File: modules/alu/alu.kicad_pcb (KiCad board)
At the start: 2 copper layers, 95 parts, among them Q1 2N3904, Q10 2N3906, Q11 2N3904, Q12 2N3904, Q13 2N3904, Q14 2N3904, Q15 2N3904, Q16 2N3904, Q17 2N3904, Q18 2N3906, Q19 2N3904, Q2 2N3904, Q20 2N3906, Q21 2N3904, Q22 2N3906, Q23 2N3904, Q24 2N3906, Q25 2N3906, Q26 2N3906, Q27 2N3906, Q28 2N3904, Q29 2N3904, Q3 2N3904, Q30 2N3904, Q31 2N3906, Q32 2N3906, Q33 2N3904, Q34 2N3904, Q35 2N3906, Q36 2N3904, Q37 2N3906, Q38 2N3906, Q39 2N3906, Q4 2N3904, Q40 2N3906, Q41 2N3906, Q42 2N3906, Q43 2N3904, Q44 2N3904, Q45 2N3904, Q5 2N3904, Q6 2N3904, Q7 2N3906, Q8 2N3906, Q9 2N3906

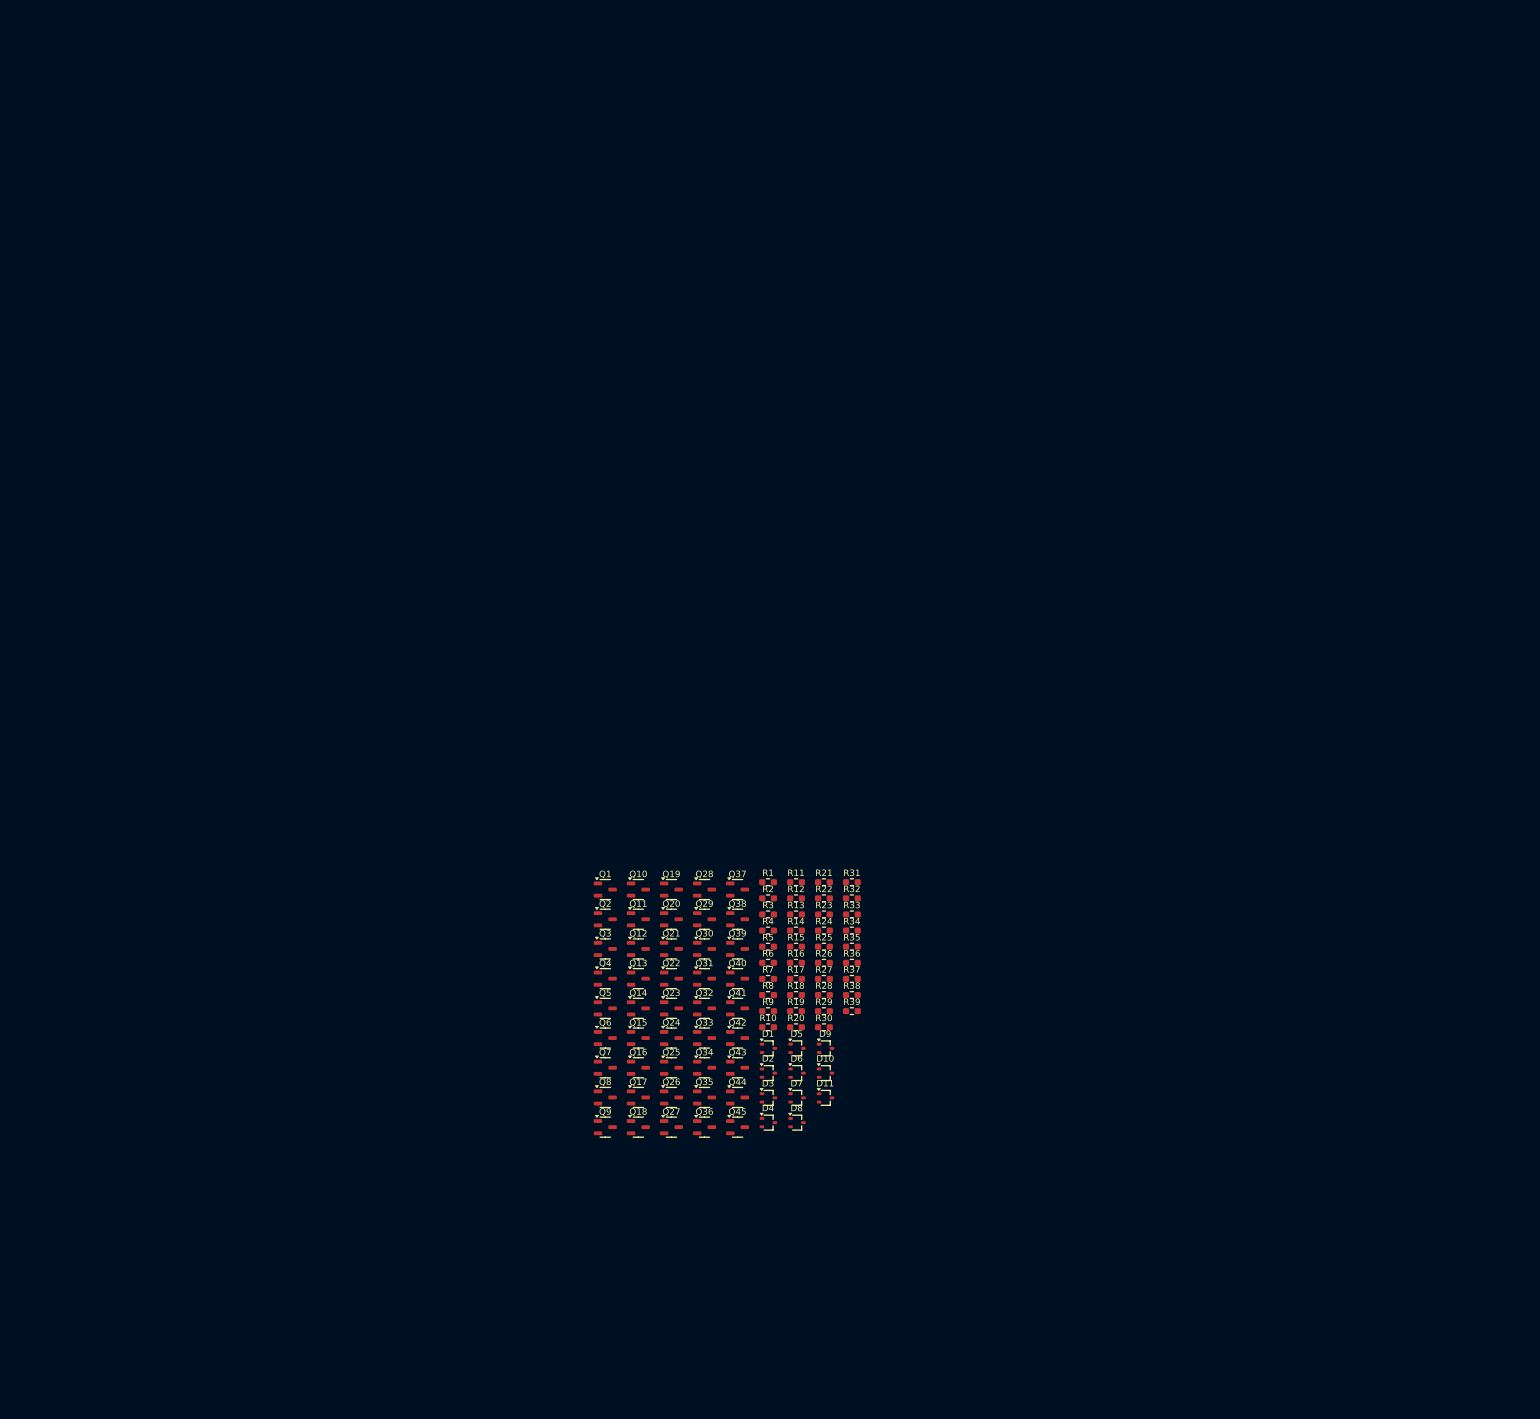
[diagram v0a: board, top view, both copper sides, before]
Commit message: Small ALU fix.
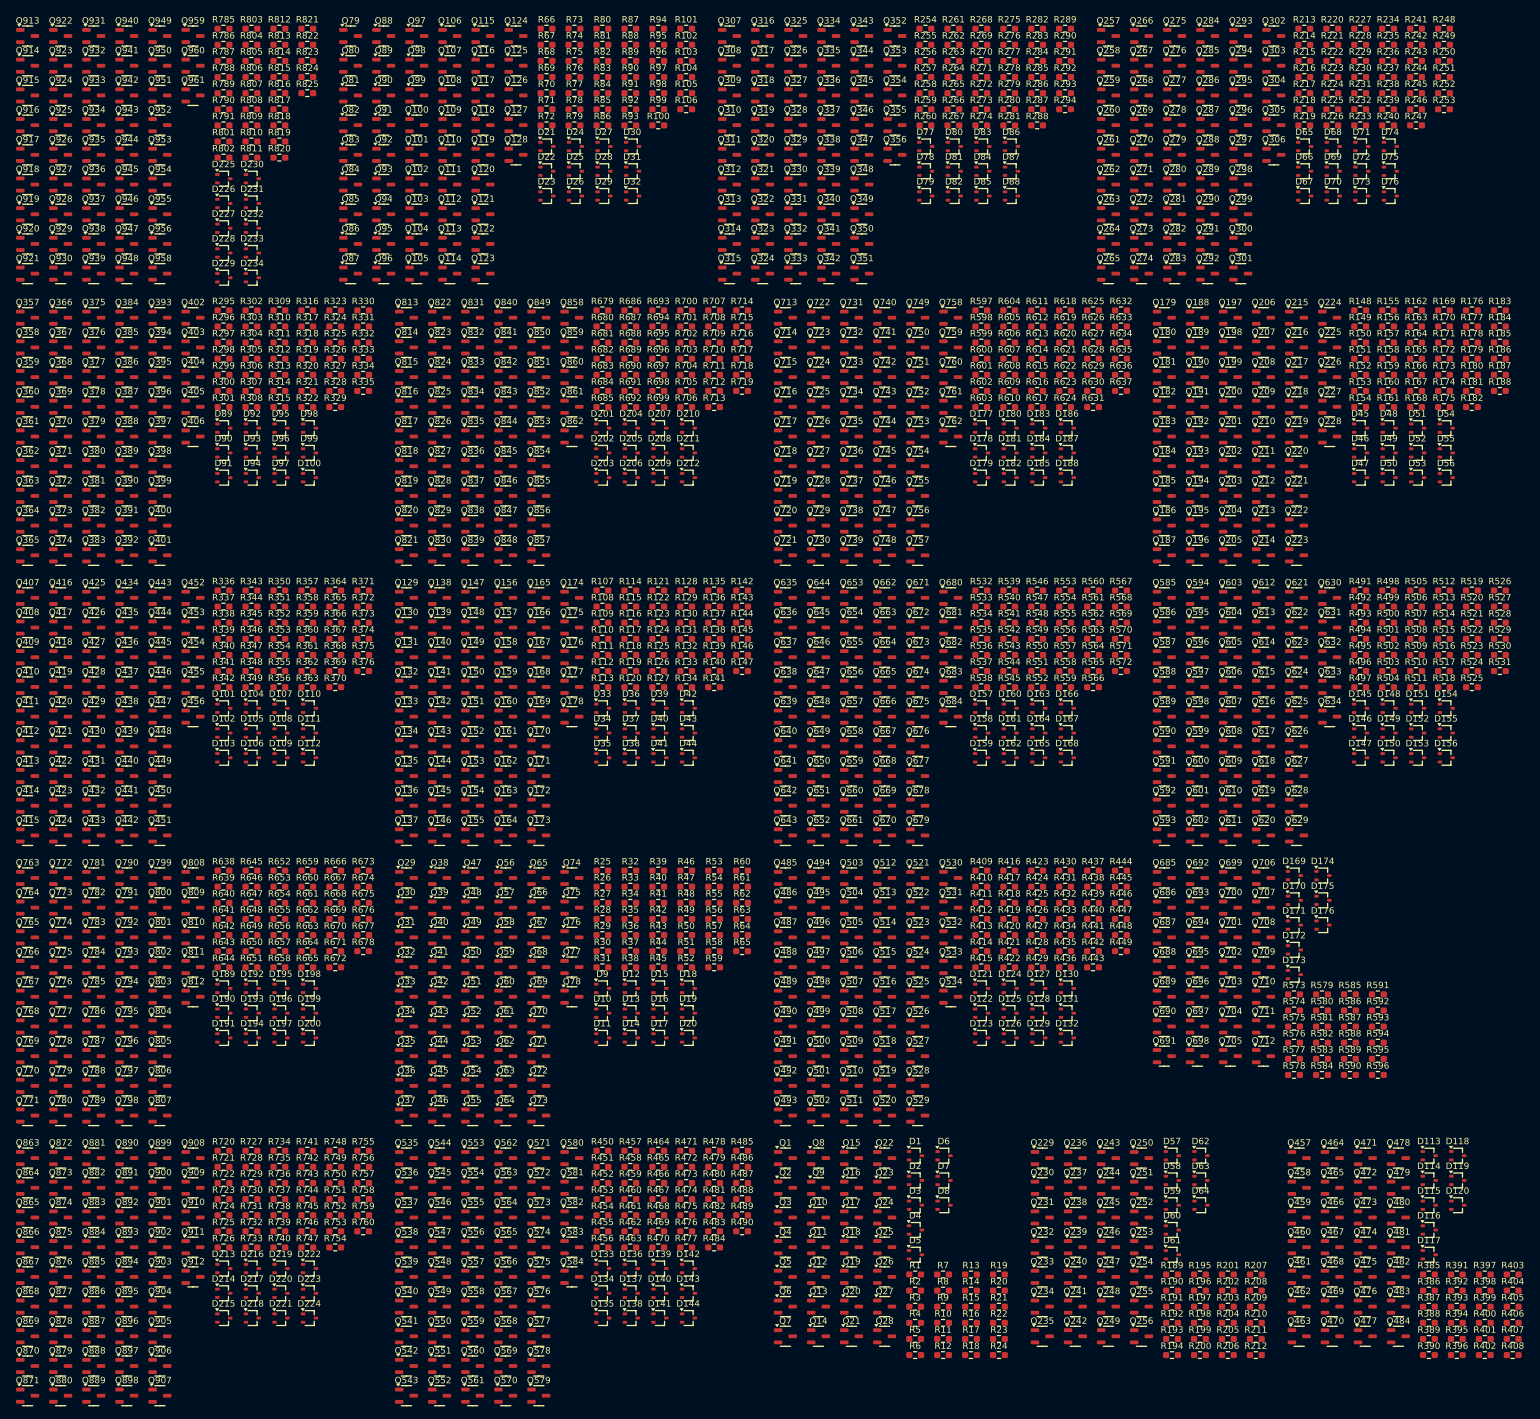
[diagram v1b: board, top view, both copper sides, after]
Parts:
- added D100: BAT54W, Package_TO_SOT_SMD:SOT-323_SC-70, F.Cu at (73.8, 3.92)
- added D101: BAT54W, Package_TO_SOT_SMD:SOT-323_SC-70, F.Cu at (60.5, 39.8)
- added D102: BAT54W, Package_TO_SOT_SMD:SOT-323_SC-70, F.Cu at (60.5, 43.7)
- added D103: BAT54W, Package_TO_SOT_SMD:SOT-323_SC-70, F.Cu at (60.5, 47.5)
- added D104: BAT54W, Package_TO_SOT_SMD:SOT-323_SC-70, F.Cu at (65.0, 39.8)
- added D105: BAT54W, Package_TO_SOT_SMD:SOT-323_SC-70, F.Cu at (65.0, 43.7)
- added D106: BAT54W, Package_TO_SOT_SMD:SOT-323_SC-70, F.Cu at (65.0, 47.5)
- added D107: BAT54W, Package_TO_SOT_SMD:SOT-323_SC-70, F.Cu at (69.4, 39.8)
- added D108: BAT54W, Package_TO_SOT_SMD:SOT-323_SC-70, F.Cu at (69.4, 43.7)
- added D109: BAT54W, Package_TO_SOT_SMD:SOT-323_SC-70, F.Cu at (69.4, 47.5)
- added D110: BAT54W, Package_TO_SOT_SMD:SOT-323_SC-70, F.Cu at (73.8, 39.8)
- added D111: BAT54W, Package_TO_SOT_SMD:SOT-323_SC-70, F.Cu at (73.8, 43.7)
- added D112: BAT54W, Package_TO_SOT_SMD:SOT-323_SC-70, F.Cu at (73.8, 47.5)
- added D113: BAT54W, Package_TO_SOT_SMD:SOT-323_SC-70, F.Cu at (248.2, 109.5)
- added D114: BAT54W, Package_TO_SOT_SMD:SOT-323_SC-70, F.Cu at (248.2, 113.4)
- added D115: BAT54W, Package_TO_SOT_SMD:SOT-323_SC-70, F.Cu at (248.2, 117.2)
- added D116: BAT54W, Package_TO_SOT_SMD:SOT-323_SC-70, F.Cu at (248.2, 121.1)
- added D117: BAT54W, Package_TO_SOT_SMD:SOT-323_SC-70, F.Cu at (248.2, 124.9)
- added D118: BAT54W, Package_TO_SOT_SMD:SOT-323_SC-70, F.Cu at (252.7, 109.5)
- added D119: BAT54W, Package_TO_SOT_SMD:SOT-323_SC-70, F.Cu at (252.7, 113.4)
- added D12: BAT54W, Package_TO_SOT_SMD:SOT-323_SC-70, F.Cu at (124.0, 83.5)
- added D120: BAT54W, Package_TO_SOT_SMD:SOT-323_SC-70, F.Cu at (252.7, 117.2)
- added D121: BAT54W, Package_TO_SOT_SMD:SOT-323_SC-70, F.Cu at (178.5, 83.5)
- added D122: BAT54W, Package_TO_SOT_SMD:SOT-323_SC-70, F.Cu at (178.5, 87.3)
- added D123: BAT54W, Package_TO_SOT_SMD:SOT-323_SC-70, F.Cu at (178.5, 91.2)
- added D124: BAT54W, Package_TO_SOT_SMD:SOT-323_SC-70, F.Cu at (182.9, 83.5)
- added D125: BAT54W, Package_TO_SOT_SMD:SOT-323_SC-70, F.Cu at (182.9, 87.3)
- added D126: BAT54W, Package_TO_SOT_SMD:SOT-323_SC-70, F.Cu at (182.9, 91.2)
- added D127: BAT54W, Package_TO_SOT_SMD:SOT-323_SC-70, F.Cu at (187.4, 83.5)
- added D128: BAT54W, Package_TO_SOT_SMD:SOT-323_SC-70, F.Cu at (187.4, 87.3)
- added D129: BAT54W, Package_TO_SOT_SMD:SOT-323_SC-70, F.Cu at (187.4, 91.2)
- added D13: BAT54W, Package_TO_SOT_SMD:SOT-323_SC-70, F.Cu at (124.0, 87.3)
- added D130: BAT54W, Package_TO_SOT_SMD:SOT-323_SC-70, F.Cu at (191.8, 83.5)
- added D131: BAT54W, Package_TO_SOT_SMD:SOT-323_SC-70, F.Cu at (191.8, 87.3)
- added D132: BAT54W, Package_TO_SOT_SMD:SOT-323_SC-70, F.Cu at (191.8, 91.2)
- added D133: BAT54W, Package_TO_SOT_SMD:SOT-323_SC-70, F.Cu at (119.5, 127.1)
- added D134: BAT54W, Package_TO_SOT_SMD:SOT-323_SC-70, F.Cu at (119.5, 130.9)
- added D135: BAT54W, Package_TO_SOT_SMD:SOT-323_SC-70, F.Cu at (119.5, 134.8)
- added D136: BAT54W, Package_TO_SOT_SMD:SOT-323_SC-70, F.Cu at (124.0, 127.1)
- added D137: BAT54W, Package_TO_SOT_SMD:SOT-323_SC-70, F.Cu at (124.0, 130.9)
- added D138: BAT54W, Package_TO_SOT_SMD:SOT-323_SC-70, F.Cu at (124.0, 134.8)
- added D139: BAT54W, Package_TO_SOT_SMD:SOT-323_SC-70, F.Cu at (128.4, 127.1)
- added D14: BAT54W, Package_TO_SOT_SMD:SOT-323_SC-70, F.Cu at (124.0, 91.2)
- added D140: BAT54W, Package_TO_SOT_SMD:SOT-323_SC-70, F.Cu at (128.4, 130.9)
- added D141: BAT54W, Package_TO_SOT_SMD:SOT-323_SC-70, F.Cu at (128.4, 134.8)
- added D142: BAT54W, Package_TO_SOT_SMD:SOT-323_SC-70, F.Cu at (132.8, 127.1)
- added D143: BAT54W, Package_TO_SOT_SMD:SOT-323_SC-70, F.Cu at (132.8, 130.9)
- added D144: BAT54W, Package_TO_SOT_SMD:SOT-323_SC-70, F.Cu at (132.8, 134.8)
- added D145: BAT54W, Package_TO_SOT_SMD:SOT-323_SC-70, F.Cu at (237.5, 39.8)
- added D146: BAT54W, Package_TO_SOT_SMD:SOT-323_SC-70, F.Cu at (237.5, 43.7)
- added D147: BAT54W, Package_TO_SOT_SMD:SOT-323_SC-70, F.Cu at (237.5, 47.5)
- added D148: BAT54W, Package_TO_SOT_SMD:SOT-323_SC-70, F.Cu at (241.9, 39.8)
- added D149: BAT54W, Package_TO_SOT_SMD:SOT-323_SC-70, F.Cu at (241.9, 43.7)
- added D15: BAT54W, Package_TO_SOT_SMD:SOT-323_SC-70, F.Cu at (128.4, 83.5)
- added D150: BAT54W, Package_TO_SOT_SMD:SOT-323_SC-70, F.Cu at (241.9, 47.5)
- added D151: BAT54W, Package_TO_SOT_SMD:SOT-323_SC-70, F.Cu at (246.4, 39.8)
- added D152: BAT54W, Package_TO_SOT_SMD:SOT-323_SC-70, F.Cu at (246.4, 43.7)
- added D153: BAT54W, Package_TO_SOT_SMD:SOT-323_SC-70, F.Cu at (246.4, 47.5)
- added D154: BAT54W, Package_TO_SOT_SMD:SOT-323_SC-70, F.Cu at (250.8, 39.8)
- added D155: BAT54W, Package_TO_SOT_SMD:SOT-323_SC-70, F.Cu at (250.8, 43.7)
- added D156: BAT54W, Package_TO_SOT_SMD:SOT-323_SC-70, F.Cu at (250.8, 47.5)
- added D157: BAT54W, Package_TO_SOT_SMD:SOT-323_SC-70, F.Cu at (178.5, 39.8)
- added D158: BAT54W, Package_TO_SOT_SMD:SOT-323_SC-70, F.Cu at (178.5, 43.7)
- added D159: BAT54W, Package_TO_SOT_SMD:SOT-323_SC-70, F.Cu at (178.5, 47.5)
- added D16: BAT54W, Package_TO_SOT_SMD:SOT-323_SC-70, F.Cu at (128.4, 87.3)
- added D160: BAT54W, Package_TO_SOT_SMD:SOT-323_SC-70, F.Cu at (182.9, 39.8)
- added D161: BAT54W, Package_TO_SOT_SMD:SOT-323_SC-70, F.Cu at (182.9, 43.7)
- added D162: BAT54W, Package_TO_SOT_SMD:SOT-323_SC-70, F.Cu at (182.9, 47.5)
- added D163: BAT54W, Package_TO_SOT_SMD:SOT-323_SC-70, F.Cu at (187.4, 39.8)
- added D164: BAT54W, Package_TO_SOT_SMD:SOT-323_SC-70, F.Cu at (187.4, 43.7)
- added D165: BAT54W, Package_TO_SOT_SMD:SOT-323_SC-70, F.Cu at (187.4, 47.5)
- added D166: BAT54W, Package_TO_SOT_SMD:SOT-323_SC-70, F.Cu at (191.8, 39.8)
- added D167: BAT54W, Package_TO_SOT_SMD:SOT-323_SC-70, F.Cu at (191.8, 43.7)
- added D168: BAT54W, Package_TO_SOT_SMD:SOT-323_SC-70, F.Cu at (191.8, 47.5)
- added D169: BAT54W, Package_TO_SOT_SMD:SOT-323_SC-70, F.Cu at (227.2, 65.9)
- added D17: BAT54W, Package_TO_SOT_SMD:SOT-323_SC-70, F.Cu at (128.4, 91.2)
- added D170: BAT54W, Package_TO_SOT_SMD:SOT-323_SC-70, F.Cu at (227.2, 69.7)
- added D171: BAT54W, Package_TO_SOT_SMD:SOT-323_SC-70, F.Cu at (227.2, 73.6)
- added D172: BAT54W, Package_TO_SOT_SMD:SOT-323_SC-70, F.Cu at (227.2, 77.5)
- added D173: BAT54W, Package_TO_SOT_SMD:SOT-323_SC-70, F.Cu at (227.2, 81.3)
- added D174: BAT54W, Package_TO_SOT_SMD:SOT-323_SC-70, F.Cu at (231.7, 65.9)
- added D175: BAT54W, Package_TO_SOT_SMD:SOT-323_SC-70, F.Cu at (231.7, 69.7)
- added D176: BAT54W, Package_TO_SOT_SMD:SOT-323_SC-70, F.Cu at (231.7, 73.6)
- added D177: BAT54W, Package_TO_SOT_SMD:SOT-323_SC-70, F.Cu at (178.5, -3.79)
- added D178: BAT54W, Package_TO_SOT_SMD:SOT-323_SC-70, F.Cu at (178.5, 0.07)
- added D179: BAT54W, Package_TO_SOT_SMD:SOT-323_SC-70, F.Cu at (178.5, 3.92)
- added D18: BAT54W, Package_TO_SOT_SMD:SOT-323_SC-70, F.Cu at (132.8, 83.5)
- added D180: BAT54W, Package_TO_SOT_SMD:SOT-323_SC-70, F.Cu at (182.9, -3.79)
- added D181: BAT54W, Package_TO_SOT_SMD:SOT-323_SC-70, F.Cu at (182.9, 0.07)
- added D182: BAT54W, Package_TO_SOT_SMD:SOT-323_SC-70, F.Cu at (182.9, 3.92)
- added D183: BAT54W, Package_TO_SOT_SMD:SOT-323_SC-70, F.Cu at (187.4, -3.79)
- added D184: BAT54W, Package_TO_SOT_SMD:SOT-323_SC-70, F.Cu at (187.4, 0.07)
- added D185: BAT54W, Package_TO_SOT_SMD:SOT-323_SC-70, F.Cu at (187.4, 3.92)
- added D186: BAT54W, Package_TO_SOT_SMD:SOT-323_SC-70, F.Cu at (191.8, -3.79)
- added D187: BAT54W, Package_TO_SOT_SMD:SOT-323_SC-70, F.Cu at (191.8, 0.07)
- added D188: BAT54W, Package_TO_SOT_SMD:SOT-323_SC-70, F.Cu at (191.8, 3.92)
- added D189: BAT54W, Package_TO_SOT_SMD:SOT-323_SC-70, F.Cu at (60.5, 83.5)
- added D19: BAT54W, Package_TO_SOT_SMD:SOT-323_SC-70, F.Cu at (132.8, 87.3)
- added D190: BAT54W, Package_TO_SOT_SMD:SOT-323_SC-70, F.Cu at (60.5, 87.3)
- added D191: BAT54W, Package_TO_SOT_SMD:SOT-323_SC-70, F.Cu at (60.5, 91.2)
- added D192: BAT54W, Package_TO_SOT_SMD:SOT-323_SC-70, F.Cu at (65.0, 83.5)
- added D193: BAT54W, Package_TO_SOT_SMD:SOT-323_SC-70, F.Cu at (65.0, 87.3)
- added D194: BAT54W, Package_TO_SOT_SMD:SOT-323_SC-70, F.Cu at (65.0, 91.2)
- added D195: BAT54W, Package_TO_SOT_SMD:SOT-323_SC-70, F.Cu at (69.4, 83.5)
- added D196: BAT54W, Package_TO_SOT_SMD:SOT-323_SC-70, F.Cu at (69.4, 87.3)
- added D197: BAT54W, Package_TO_SOT_SMD:SOT-323_SC-70, F.Cu at (69.4, 91.2)
- added D198: BAT54W, Package_TO_SOT_SMD:SOT-323_SC-70, F.Cu at (73.8, 83.5)
- added D199: BAT54W, Package_TO_SOT_SMD:SOT-323_SC-70, F.Cu at (73.8, 87.3)
- added D20: BAT54W, Package_TO_SOT_SMD:SOT-323_SC-70, F.Cu at (132.8, 91.2)
- added D200: BAT54W, Package_TO_SOT_SMD:SOT-323_SC-70, F.Cu at (73.8, 91.2)
- added D201: BAT54W, Package_TO_SOT_SMD:SOT-323_SC-70, F.Cu at (119.5, -3.79)
- added D202: BAT54W, Package_TO_SOT_SMD:SOT-323_SC-70, F.Cu at (119.5, 0.07)
- added D203: BAT54W, Package_TO_SOT_SMD:SOT-323_SC-70, F.Cu at (119.5, 3.92)
- added D204: BAT54W, Package_TO_SOT_SMD:SOT-323_SC-70, F.Cu at (124.0, -3.79)
- added D205: BAT54W, Package_TO_SOT_SMD:SOT-323_SC-70, F.Cu at (124.0, 0.07)
- added D206: BAT54W, Package_TO_SOT_SMD:SOT-323_SC-70, F.Cu at (124.0, 3.92)
- added D207: BAT54W, Package_TO_SOT_SMD:SOT-323_SC-70, F.Cu at (128.4, -3.79)
- added D208: BAT54W, Package_TO_SOT_SMD:SOT-323_SC-70, F.Cu at (128.4, 0.07)
- added D209: BAT54W, Package_TO_SOT_SMD:SOT-323_SC-70, F.Cu at (128.4, 3.92)
- added D21: BAT54W, Package_TO_SOT_SMD:SOT-323_SC-70, F.Cu at (110.8, -47.6)
- added D210: BAT54W, Package_TO_SOT_SMD:SOT-323_SC-70, F.Cu at (132.8, -3.79)
- added D211: BAT54W, Package_TO_SOT_SMD:SOT-323_SC-70, F.Cu at (132.8, 0.07)
- added D212: BAT54W, Package_TO_SOT_SMD:SOT-323_SC-70, F.Cu at (132.8, 3.92)
- added D213: BAT54W, Package_TO_SOT_SMD:SOT-323_SC-70, F.Cu at (60.5, 127.1)
- added D214: BAT54W, Package_TO_SOT_SMD:SOT-323_SC-70, F.Cu at (60.5, 130.9)
- added D215: BAT54W, Package_TO_SOT_SMD:SOT-323_SC-70, F.Cu at (60.5, 134.8)
- added D216: BAT54W, Package_TO_SOT_SMD:SOT-323_SC-70, F.Cu at (65.0, 127.1)
- added D217: BAT54W, Package_TO_SOT_SMD:SOT-323_SC-70, F.Cu at (65.0, 130.9)
- added D218: BAT54W, Package_TO_SOT_SMD:SOT-323_SC-70, F.Cu at (65.0, 134.8)
- added D219: BAT54W, Package_TO_SOT_SMD:SOT-323_SC-70, F.Cu at (69.4, 127.1)
- added D22: BAT54W, Package_TO_SOT_SMD:SOT-323_SC-70, F.Cu at (110.8, -43.8)
- added D220: BAT54W, Package_TO_SOT_SMD:SOT-323_SC-70, F.Cu at (69.4, 130.9)
- added D221: BAT54W, Package_TO_SOT_SMD:SOT-323_SC-70, F.Cu at (69.4, 134.8)
- added D222: BAT54W, Package_TO_SOT_SMD:SOT-323_SC-70, F.Cu at (73.8, 127.1)
- added D223: BAT54W, Package_TO_SOT_SMD:SOT-323_SC-70, F.Cu at (73.8, 130.9)
- added D224: BAT54W, Package_TO_SOT_SMD:SOT-323_SC-70, F.Cu at (73.8, 134.8)
- added D225: BAT54W, Package_TO_SOT_SMD:SOT-323_SC-70, F.Cu at (60.5, -42.6)
- added D226: BAT54W, Package_TO_SOT_SMD:SOT-323_SC-70, F.Cu at (60.5, -38.8)
- added D227: BAT54W, Package_TO_SOT_SMD:SOT-323_SC-70, F.Cu at (60.5, -34.9)
- added D228: BAT54W, Package_TO_SOT_SMD:SOT-323_SC-70, F.Cu at (60.5, -31.1)
- added D229: BAT54W, Package_TO_SOT_SMD:SOT-323_SC-70, F.Cu at (60.5, -27.2)
- added D23: BAT54W, Package_TO_SOT_SMD:SOT-323_SC-70, F.Cu at (110.8, -39.9)
- added D230: BAT54W, Package_TO_SOT_SMD:SOT-323_SC-70, F.Cu at (65.0, -42.6)
- added D231: BAT54W, Package_TO_SOT_SMD:SOT-323_SC-70, F.Cu at (65.0, -38.8)
- added D232: BAT54W, Package_TO_SOT_SMD:SOT-323_SC-70, F.Cu at (65.0, -34.9)
- added D233: BAT54W, Package_TO_SOT_SMD:SOT-323_SC-70, F.Cu at (65.0, -31.1)
- added D234: BAT54W, Package_TO_SOT_SMD:SOT-323_SC-70, F.Cu at (65.0, -27.2)
- added D24: BAT54W, Package_TO_SOT_SMD:SOT-323_SC-70, F.Cu at (115.2, -47.6)
- added D25: BAT54W, Package_TO_SOT_SMD:SOT-323_SC-70, F.Cu at (115.2, -43.8)
- added D26: BAT54W, Package_TO_SOT_SMD:SOT-323_SC-70, F.Cu at (115.2, -39.9)
- added D27: BAT54W, Package_TO_SOT_SMD:SOT-323_SC-70, F.Cu at (119.7, -47.6)
- added D28: BAT54W, Package_TO_SOT_SMD:SOT-323_SC-70, F.Cu at (119.7, -43.8)
- added D29: BAT54W, Package_TO_SOT_SMD:SOT-323_SC-70, F.Cu at (119.7, -39.9)
- added D30: BAT54W, Package_TO_SOT_SMD:SOT-323_SC-70, F.Cu at (124.2, -47.6)
- added D31: BAT54W, Package_TO_SOT_SMD:SOT-323_SC-70, F.Cu at (124.2, -43.8)
- added D32: BAT54W, Package_TO_SOT_SMD:SOT-323_SC-70, F.Cu at (124.2, -39.9)
- added D33: BAT54W, Package_TO_SOT_SMD:SOT-323_SC-70, F.Cu at (119.5, 39.8)
- added D34: BAT54W, Package_TO_SOT_SMD:SOT-323_SC-70, F.Cu at (119.5, 43.7)
- added D35: BAT54W, Package_TO_SOT_SMD:SOT-323_SC-70, F.Cu at (119.5, 47.5)
- added D36: BAT54W, Package_TO_SOT_SMD:SOT-323_SC-70, F.Cu at (124.0, 39.8)
- added D37: BAT54W, Package_TO_SOT_SMD:SOT-323_SC-70, F.Cu at (124.0, 43.7)
- added D38: BAT54W, Package_TO_SOT_SMD:SOT-323_SC-70, F.Cu at (124.0, 47.5)
- added D39: BAT54W, Package_TO_SOT_SMD:SOT-323_SC-70, F.Cu at (128.4, 39.8)
- added D40: BAT54W, Package_TO_SOT_SMD:SOT-323_SC-70, F.Cu at (128.4, 43.7)
- added D41: BAT54W, Package_TO_SOT_SMD:SOT-323_SC-70, F.Cu at (128.4, 47.5)
- added D42: BAT54W, Package_TO_SOT_SMD:SOT-323_SC-70, F.Cu at (132.8, 39.8)
- added D43: BAT54W, Package_TO_SOT_SMD:SOT-323_SC-70, F.Cu at (132.8, 43.7)
- added D44: BAT54W, Package_TO_SOT_SMD:SOT-323_SC-70, F.Cu at (132.8, 47.5)
- added D45: BAT54W, Package_TO_SOT_SMD:SOT-323_SC-70, F.Cu at (237.5, -3.79)
- added D46: BAT54W, Package_TO_SOT_SMD:SOT-323_SC-70, F.Cu at (237.5, 0.07)
- added D47: BAT54W, Package_TO_SOT_SMD:SOT-323_SC-70, F.Cu at (237.5, 3.92)
- added D48: BAT54W, Package_TO_SOT_SMD:SOT-323_SC-70, F.Cu at (241.9, -3.79)
- added D49: BAT54W, Package_TO_SOT_SMD:SOT-323_SC-70, F.Cu at (241.9, 0.07)
- added D50: BAT54W, Package_TO_SOT_SMD:SOT-323_SC-70, F.Cu at (241.9, 3.92)
- added D51: BAT54W, Package_TO_SOT_SMD:SOT-323_SC-70, F.Cu at (246.4, -3.79)
- added D52: BAT54W, Package_TO_SOT_SMD:SOT-323_SC-70, F.Cu at (246.4, 0.07)
- added D53: BAT54W, Package_TO_SOT_SMD:SOT-323_SC-70, F.Cu at (246.4, 3.92)
- added D54: BAT54W, Package_TO_SOT_SMD:SOT-323_SC-70, F.Cu at (250.8, -3.79)
- added D55: BAT54W, Package_TO_SOT_SMD:SOT-323_SC-70, F.Cu at (250.8, 0.07)
- added D56: BAT54W, Package_TO_SOT_SMD:SOT-323_SC-70, F.Cu at (250.8, 3.92)
- added D57: BAT54W, Package_TO_SOT_SMD:SOT-323_SC-70, F.Cu at (208.2, 109.5)
- added D58: BAT54W, Package_TO_SOT_SMD:SOT-323_SC-70, F.Cu at (208.2, 113.4)
- added D59: BAT54W, Package_TO_SOT_SMD:SOT-323_SC-70, F.Cu at (208.2, 117.2)
- added D60: BAT54W, Package_TO_SOT_SMD:SOT-323_SC-70, F.Cu at (208.2, 121.1)
- added D61: BAT54W, Package_TO_SOT_SMD:SOT-323_SC-70, F.Cu at (208.2, 124.9)
- added D62: BAT54W, Package_TO_SOT_SMD:SOT-323_SC-70, F.Cu at (212.7, 109.5)
- added D63: BAT54W, Package_TO_SOT_SMD:SOT-323_SC-70, F.Cu at (212.7, 113.4)
- added D64: BAT54W, Package_TO_SOT_SMD:SOT-323_SC-70, F.Cu at (212.7, 117.2)
- added D65: BAT54W, Package_TO_SOT_SMD:SOT-323_SC-70, F.Cu at (228.8, -47.6)
- added D66: BAT54W, Package_TO_SOT_SMD:SOT-323_SC-70, F.Cu at (228.8, -43.8)
- added D67: BAT54W, Package_TO_SOT_SMD:SOT-323_SC-70, F.Cu at (228.8, -39.9)
- added D68: BAT54W, Package_TO_SOT_SMD:SOT-323_SC-70, F.Cu at (233.2, -47.6)
- added D69: BAT54W, Package_TO_SOT_SMD:SOT-323_SC-70, F.Cu at (233.2, -43.8)
- added D70: BAT54W, Package_TO_SOT_SMD:SOT-323_SC-70, F.Cu at (233.2, -39.9)
- added D71: BAT54W, Package_TO_SOT_SMD:SOT-323_SC-70, F.Cu at (237.7, -47.6)
- added D72: BAT54W, Package_TO_SOT_SMD:SOT-323_SC-70, F.Cu at (237.7, -43.8)
- added D73: BAT54W, Package_TO_SOT_SMD:SOT-323_SC-70, F.Cu at (237.7, -39.9)
- added D74: BAT54W, Package_TO_SOT_SMD:SOT-323_SC-70, F.Cu at (242.2, -47.6)
- added D75: BAT54W, Package_TO_SOT_SMD:SOT-323_SC-70, F.Cu at (242.2, -43.8)
- added D76: BAT54W, Package_TO_SOT_SMD:SOT-323_SC-70, F.Cu at (242.2, -39.9)
- added D77: BAT54W, Package_TO_SOT_SMD:SOT-323_SC-70, F.Cu at (169.8, -47.6)
- added D78: BAT54W, Package_TO_SOT_SMD:SOT-323_SC-70, F.Cu at (169.8, -43.8)
- added D79: BAT54W, Package_TO_SOT_SMD:SOT-323_SC-70, F.Cu at (169.8, -39.9)
- added D80: BAT54W, Package_TO_SOT_SMD:SOT-323_SC-70, F.Cu at (174.2, -47.6)
- added D81: BAT54W, Package_TO_SOT_SMD:SOT-323_SC-70, F.Cu at (174.2, -43.8)
- added D82: BAT54W, Package_TO_SOT_SMD:SOT-323_SC-70, F.Cu at (174.2, -39.9)
- added D83: BAT54W, Package_TO_SOT_SMD:SOT-323_SC-70, F.Cu at (178.7, -47.6)
- added D84: BAT54W, Package_TO_SOT_SMD:SOT-323_SC-70, F.Cu at (178.7, -43.8)
- added D85: BAT54W, Package_TO_SOT_SMD:SOT-323_SC-70, F.Cu at (178.7, -39.9)
- added D86: BAT54W, Package_TO_SOT_SMD:SOT-323_SC-70, F.Cu at (183.2, -47.6)
- added D87: BAT54W, Package_TO_SOT_SMD:SOT-323_SC-70, F.Cu at (183.2, -43.8)
- added D88: BAT54W, Package_TO_SOT_SMD:SOT-323_SC-70, F.Cu at (183.2, -39.9)
- added D89: BAT54W, Package_TO_SOT_SMD:SOT-323_SC-70, F.Cu at (60.5, -3.79)
- added D90: BAT54W, Package_TO_SOT_SMD:SOT-323_SC-70, F.Cu at (60.5, 0.07)
- added D91: BAT54W, Package_TO_SOT_SMD:SOT-323_SC-70, F.Cu at (60.5, 3.92)
- added D92: BAT54W, Package_TO_SOT_SMD:SOT-323_SC-70, F.Cu at (65.0, -3.79)
- added D93: BAT54W, Package_TO_SOT_SMD:SOT-323_SC-70, F.Cu at (65.0, 0.07)
- added D94: BAT54W, Package_TO_SOT_SMD:SOT-323_SC-70, F.Cu at (65.0, 3.92)
- added D95: BAT54W, Package_TO_SOT_SMD:SOT-323_SC-70, F.Cu at (69.4, -3.79)
- added D96: BAT54W, Package_TO_SOT_SMD:SOT-323_SC-70, F.Cu at (69.4, 0.07)
- added D97: BAT54W, Package_TO_SOT_SMD:SOT-323_SC-70, F.Cu at (69.4, 3.92)
- added D98: BAT54W, Package_TO_SOT_SMD:SOT-323_SC-70, F.Cu at (73.8, -3.79)
- added D99: BAT54W, Package_TO_SOT_SMD:SOT-323_SC-70, F.Cu at (73.8, 0.07)
- added Q100: 2N3904, Package_TO_SOT_SMD:SOT-23-3, F.Cu at (90.5, -51.0)
- added Q101: 2N3904, Package_TO_SOT_SMD:SOT-23-3, F.Cu at (90.5, -46.3)
- added Q102: 2N3904, Package_TO_SOT_SMD:SOT-23-3, F.Cu at (90.5, -41.7)
- added Q103: 2N3906, Package_TO_SOT_SMD:SOT-23-3, F.Cu at (90.5, -37.1)
- added Q104: 2N3904, Package_TO_SOT_SMD:SOT-23-3, F.Cu at (90.5, -32.5)
- added Q105: 2N3906, Package_TO_SOT_SMD:SOT-23-3, F.Cu at (90.5, -27.8)
- added Q106: 2N3904, Package_TO_SOT_SMD:SOT-23-3, F.Cu at (95.7, -64.8)
- added Q107: 2N3906, Package_TO_SOT_SMD:SOT-23-3, F.Cu at (95.7, -60.2)
- added Q108: 2N3904, Package_TO_SOT_SMD:SOT-23-3, F.Cu at (95.7, -55.6)
- added Q109: 2N3906, Package_TO_SOT_SMD:SOT-23-3, F.Cu at (95.7, -51.0)
- added Q110: 2N3906, Package_TO_SOT_SMD:SOT-23-3, F.Cu at (95.7, -46.3)
- added Q111: 2N3906, Package_TO_SOT_SMD:SOT-23-3, F.Cu at (95.7, -41.7)
- added Q112: 2N3904, Package_TO_SOT_SMD:SOT-23-3, F.Cu at (95.7, -37.1)
- added Q113: 2N3906, Package_TO_SOT_SMD:SOT-23-3, F.Cu at (95.7, -32.5)
- added Q114: 2N3906, Package_TO_SOT_SMD:SOT-23-3, F.Cu at (95.7, -27.8)
- added Q115: 2N3906, Package_TO_SOT_SMD:SOT-23-3, F.Cu at (100.8, -64.8)
- added Q116: 2N3906, Package_TO_SOT_SMD:SOT-23-3, F.Cu at (100.8, -60.2)
- added Q117: 2N3904, Package_TO_SOT_SMD:SOT-23-3, F.Cu at (100.8, -55.6)
- added Q118: 2N3906, Package_TO_SOT_SMD:SOT-23-3, F.Cu at (100.8, -51.0)
- added Q119: 2N3906, Package_TO_SOT_SMD:SOT-23-3, F.Cu at (100.8, -46.3)
- added Q120: 2N3906, Package_TO_SOT_SMD:SOT-23-3, F.Cu at (100.8, -41.7)
- added Q121: 2N3906, Package_TO_SOT_SMD:SOT-23-3, F.Cu at (100.8, -37.1)
- added Q122: 2N3904, Package_TO_SOT_SMD:SOT-23-3, F.Cu at (100.8, -32.5)
- added Q123: 2N3904, Package_TO_SOT_SMD:SOT-23-3, F.Cu at (100.8, -27.8)
- added Q124: 2N3904, Package_TO_SOT_SMD:SOT-23-3, F.Cu at (106.0, -64.8)
- added Q125: 2N3904, Package_TO_SOT_SMD:SOT-23-3, F.Cu at (106.0, -60.2)
- added Q126: 2N3904, Package_TO_SOT_SMD:SOT-23-3, F.Cu at (106.0, -55.6)
- added Q127: 2N3904, Package_TO_SOT_SMD:SOT-23-3, F.Cu at (106.0, -51.0)
- added Q128: 2N3904, Package_TO_SOT_SMD:SOT-23-3, F.Cu at (106.0, -46.3)
- added Q129: 2N3904, Package_TO_SOT_SMD:SOT-23-3, F.Cu at (89.0, 22.6)
- added Q130: 2N3904, Package_TO_SOT_SMD:SOT-23-3, F.Cu at (89.0, 27.3)
- added Q131: 2N3904, Package_TO_SOT_SMD:SOT-23-3, F.Cu at (89.0, 31.9)
- added Q132: 2N3904, Package_TO_SOT_SMD:SOT-23-3, F.Cu at (89.0, 36.5)
- added Q133: 2N3904, Package_TO_SOT_SMD:SOT-23-3, F.Cu at (89.0, 41.1)
- added Q134: 2N3904, Package_TO_SOT_SMD:SOT-23-3, F.Cu at (89.0, 45.8)
- added Q135: 2N3904, Package_TO_SOT_SMD:SOT-23-3, F.Cu at (89.0, 50.4)
- added Q136: 2N3904, Package_TO_SOT_SMD:SOT-23-3, F.Cu at (89.0, 55.0)
- added Q137: 2N3906, Package_TO_SOT_SMD:SOT-23-3, F.Cu at (89.0, 59.6)
- added Q138: 2N3906, Package_TO_SOT_SMD:SOT-23-3, F.Cu at (94.1, 22.6)
- added Q139: 2N3906, Package_TO_SOT_SMD:SOT-23-3, F.Cu at (94.1, 27.3)
- added Q140: 2N3906, Package_TO_SOT_SMD:SOT-23-3, F.Cu at (94.1, 31.9)
- added Q141: 2N3904, Package_TO_SOT_SMD:SOT-23-3, F.Cu at (94.1, 36.5)
- added Q142: 2N3904, Package_TO_SOT_SMD:SOT-23-3, F.Cu at (94.1, 41.1)
- added Q143: 2N3904, Package_TO_SOT_SMD:SOT-23-3, F.Cu at (94.1, 45.8)
- added Q144: 2N3906, Package_TO_SOT_SMD:SOT-23-3, F.Cu at (94.1, 50.4)
- added Q145: 2N3904, Package_TO_SOT_SMD:SOT-23-3, F.Cu at (94.1, 55.0)
- added Q146: 2N3904, Package_TO_SOT_SMD:SOT-23-3, F.Cu at (94.1, 59.6)
- added Q147: 2N3906, Package_TO_SOT_SMD:SOT-23-3, F.Cu at (99.2, 22.6)
- added Q148: 2N3904, Package_TO_SOT_SMD:SOT-23-3, F.Cu at (99.2, 27.3)
- added Q149: 2N3904, Package_TO_SOT_SMD:SOT-23-3, F.Cu at (99.2, 31.9)
- added Q150: 2N3904, Package_TO_SOT_SMD:SOT-23-3, F.Cu at (99.2, 36.5)
- added Q151: 2N3904, Package_TO_SOT_SMD:SOT-23-3, F.Cu at (99.2, 41.1)
- added Q152: 2N3904, Package_TO_SOT_SMD:SOT-23-3, F.Cu at (99.2, 45.8)
- added Q153: 2N3906, Package_TO_SOT_SMD:SOT-23-3, F.Cu at (99.2, 50.4)
- added Q154: 2N3904, Package_TO_SOT_SMD:SOT-23-3, F.Cu at (99.2, 55.0)
- added Q155: 2N3906, Package_TO_SOT_SMD:SOT-23-3, F.Cu at (99.2, 59.6)
- added Q156: 2N3904, Package_TO_SOT_SMD:SOT-23-3, F.Cu at (104.4, 22.6)
- added Q157: 2N3906, Package_TO_SOT_SMD:SOT-23-3, F.Cu at (104.4, 27.3)
- added Q158: 2N3904, Package_TO_SOT_SMD:SOT-23-3, F.Cu at (104.4, 31.9)
- added Q159: 2N3906, Package_TO_SOT_SMD:SOT-23-3, F.Cu at (104.4, 36.5)
- added Q160: 2N3906, Package_TO_SOT_SMD:SOT-23-3, F.Cu at (104.4, 41.1)
- added Q161: 2N3906, Package_TO_SOT_SMD:SOT-23-3, F.Cu at (104.4, 45.8)
- added Q162: 2N3904, Package_TO_SOT_SMD:SOT-23-3, F.Cu at (104.4, 50.4)
- added Q163: 2N3906, Package_TO_SOT_SMD:SOT-23-3, F.Cu at (104.4, 55.0)
- added Q164: 2N3906, Package_TO_SOT_SMD:SOT-23-3, F.Cu at (104.4, 59.6)
- added Q165: 2N3906, Package_TO_SOT_SMD:SOT-23-3, F.Cu at (109.5, 22.6)
- added Q166: 2N3906, Package_TO_SOT_SMD:SOT-23-3, F.Cu at (109.5, 27.3)
- added Q167: 2N3904, Package_TO_SOT_SMD:SOT-23-3, F.Cu at (109.5, 31.9)
- added Q168: 2N3906, Package_TO_SOT_SMD:SOT-23-3, F.Cu at (109.5, 36.5)
- added Q169: 2N3906, Package_TO_SOT_SMD:SOT-23-3, F.Cu at (109.5, 41.1)
- added Q170: 2N3906, Package_TO_SOT_SMD:SOT-23-3, F.Cu at (109.5, 45.8)
- added Q171: 2N3906, Package_TO_SOT_SMD:SOT-23-3, F.Cu at (109.5, 50.4)
- added Q172: 2N3904, Package_TO_SOT_SMD:SOT-23-3, F.Cu at (109.5, 55.0)
- added Q173: 2N3904, Package_TO_SOT_SMD:SOT-23-3, F.Cu at (109.5, 59.6)
- added Q174: 2N3904, Package_TO_SOT_SMD:SOT-23-3, F.Cu at (114.7, 22.6)
- added Q175: 2N3904, Package_TO_SOT_SMD:SOT-23-3, F.Cu at (114.7, 27.3)
- added Q176: 2N3904, Package_TO_SOT_SMD:SOT-23-3, F.Cu at (114.7, 31.9)
- added Q177: 2N3904, Package_TO_SOT_SMD:SOT-23-3, F.Cu at (114.7, 36.5)
- added Q178: 2N3904, Package_TO_SOT_SMD:SOT-23-3, F.Cu at (114.7, 41.1)
- added Q179: 2N3904, Package_TO_SOT_SMD:SOT-23-3, F.Cu at (206.9, -21.0)
- added Q180: 2N3904, Package_TO_SOT_SMD:SOT-23-3, F.Cu at (206.9, -16.4)
- added Q181: 2N3904, Package_TO_SOT_SMD:SOT-23-3, F.Cu at (206.9, -11.7)
- added Q182: 2N3904, Package_TO_SOT_SMD:SOT-23-3, F.Cu at (206.9, -7.11)
- added Q183: 2N3904, Package_TO_SOT_SMD:SOT-23-3, F.Cu at (206.9, -2.48)
- added Q184: 2N3904, Package_TO_SOT_SMD:SOT-23-3, F.Cu at (206.9, 2.14)
- added Q185: 2N3904, Package_TO_SOT_SMD:SOT-23-3, F.Cu at (206.9, 6.76)
- added Q186: 2N3904, Package_TO_SOT_SMD:SOT-23-3, F.Cu at (206.9, 11.4)
- added Q187: 2N3906, Package_TO_SOT_SMD:SOT-23-3, F.Cu at (206.9, 16.0)
- added Q188: 2N3906, Package_TO_SOT_SMD:SOT-23-3, F.Cu at (212.1, -21.0)
- added Q189: 2N3906, Package_TO_SOT_SMD:SOT-23-3, F.Cu at (212.1, -16.4)
- added Q190: 2N3906, Package_TO_SOT_SMD:SOT-23-3, F.Cu at (212.1, -11.7)
- added Q191: 2N3904, Package_TO_SOT_SMD:SOT-23-3, F.Cu at (212.1, -7.11)
- added Q192: 2N3904, Package_TO_SOT_SMD:SOT-23-3, F.Cu at (212.1, -2.48)
- added Q193: 2N3904, Package_TO_SOT_SMD:SOT-23-3, F.Cu at (212.1, 2.14)
- added Q194: 2N3906, Package_TO_SOT_SMD:SOT-23-3, F.Cu at (212.1, 6.76)
- added Q195: 2N3904, Package_TO_SOT_SMD:SOT-23-3, F.Cu at (212.1, 11.4)
- added Q196: 2N3904, Package_TO_SOT_SMD:SOT-23-3, F.Cu at (212.1, 16.0)
- added Q197: 2N3906, Package_TO_SOT_SMD:SOT-23-3, F.Cu at (217.2, -21.0)
- added Q198: 2N3904, Package_TO_SOT_SMD:SOT-23-3, F.Cu at (217.2, -16.4)
- added Q199: 2N3904, Package_TO_SOT_SMD:SOT-23-3, F.Cu at (217.2, -11.7)
- added Q200: 2N3904, Package_TO_SOT_SMD:SOT-23-3, F.Cu at (217.2, -7.11)
- added Q201: 2N3904, Package_TO_SOT_SMD:SOT-23-3, F.Cu at (217.2, -2.48)
- added Q202: 2N3904, Package_TO_SOT_SMD:SOT-23-3, F.Cu at (217.2, 2.14)
- added Q203: 2N3906, Package_TO_SOT_SMD:SOT-23-3, F.Cu at (217.2, 6.76)
- added Q204: 2N3904, Package_TO_SOT_SMD:SOT-23-3, F.Cu at (217.2, 11.4)
- added Q205: 2N3906, Package_TO_SOT_SMD:SOT-23-3, F.Cu at (217.2, 16.0)
- added Q206: 2N3904, Package_TO_SOT_SMD:SOT-23-3, F.Cu at (222.4, -21.0)
- added Q207: 2N3906, Package_TO_SOT_SMD:SOT-23-3, F.Cu at (222.4, -16.4)
- added Q208: 2N3904, Package_TO_SOT_SMD:SOT-23-3, F.Cu at (222.4, -11.7)
- added Q209: 2N3906, Package_TO_SOT_SMD:SOT-23-3, F.Cu at (222.4, -7.11)
- added Q210: 2N3906, Package_TO_SOT_SMD:SOT-23-3, F.Cu at (222.4, -2.48)
- added Q211: 2N3906, Package_TO_SOT_SMD:SOT-23-3, F.Cu at (222.4, 2.14)
- added Q212: 2N3904, Package_TO_SOT_SMD:SOT-23-3, F.Cu at (222.4, 6.76)
- added Q213: 2N3906, Package_TO_SOT_SMD:SOT-23-3, F.Cu at (222.4, 11.4)
- added Q214: 2N3906, Package_TO_SOT_SMD:SOT-23-3, F.Cu at (222.4, 16.0)
- added Q215: 2N3906, Package_TO_SOT_SMD:SOT-23-3, F.Cu at (227.6, -21.0)
- added Q216: 2N3906, Package_TO_SOT_SMD:SOT-23-3, F.Cu at (227.6, -16.4)
- added Q217: 2N3904, Package_TO_SOT_SMD:SOT-23-3, F.Cu at (227.6, -11.7)
- added Q218: 2N3906, Package_TO_SOT_SMD:SOT-23-3, F.Cu at (227.6, -7.11)
- added Q219: 2N3906, Package_TO_SOT_SMD:SOT-23-3, F.Cu at (227.6, -2.48)
- added Q220: 2N3906, Package_TO_SOT_SMD:SOT-23-3, F.Cu at (227.6, 2.14)
- added Q221: 2N3906, Package_TO_SOT_SMD:SOT-23-3, F.Cu at (227.6, 6.76)
- added Q222: 2N3904, Package_TO_SOT_SMD:SOT-23-3, F.Cu at (227.6, 11.4)
- added Q223: 2N3904, Package_TO_SOT_SMD:SOT-23-3, F.Cu at (227.6, 16.0)
- added Q224: 2N3904, Package_TO_SOT_SMD:SOT-23-3, F.Cu at (232.7, -21.0)
- added Q225: 2N3904, Package_TO_SOT_SMD:SOT-23-3, F.Cu at (232.7, -16.4)
- added Q226: 2N3904, Package_TO_SOT_SMD:SOT-23-3, F.Cu at (232.7, -11.7)
- added Q227: 2N3904, Package_TO_SOT_SMD:SOT-23-3, F.Cu at (232.7, -7.11)
- added Q228: 2N3904, Package_TO_SOT_SMD:SOT-23-3, F.Cu at (232.7, -2.48)
- added Q229: 2N3906, Package_TO_SOT_SMD:SOT-23-3, F.Cu at (187.9, 109.9)
- added Q230: 2N3906, Package_TO_SOT_SMD:SOT-23-3, F.Cu at (187.9, 114.5)
- added Q231: 2N3906, Package_TO_SOT_SMD:SOT-23-3, F.Cu at (187.9, 119.1)
- added Q232: 2N3906, Package_TO_SOT_SMD:SOT-23-3, F.Cu at (187.9, 123.8)
- added Q233: 2N3906, Package_TO_SOT_SMD:SOT-23-3, F.Cu at (187.9, 128.4)
- added Q234: 2N3906, Package_TO_SOT_SMD:SOT-23-3, F.Cu at (187.9, 133.0)
- added Q235: 2N3906, Package_TO_SOT_SMD:SOT-23-3, F.Cu at (187.9, 137.6)
- added Q236: 2N3906, Package_TO_SOT_SMD:SOT-23-3, F.Cu at (193.1, 109.9)
- added Q237: 2N3904, Package_TO_SOT_SMD:SOT-23-3, F.Cu at (193.1, 114.5)
- added Q238: 2N3904, Package_TO_SOT_SMD:SOT-23-3, F.Cu at (193.1, 119.1)
- added Q239: 2N3904, Package_TO_SOT_SMD:SOT-23-3, F.Cu at (193.1, 123.8)
- added Q240: 2N3904, Package_TO_SOT_SMD:SOT-23-3, F.Cu at (193.1, 128.4)
- added Q241: 2N3904, Package_TO_SOT_SMD:SOT-23-3, F.Cu at (193.1, 133.0)
- added Q242: 2N3904, Package_TO_SOT_SMD:SOT-23-3, F.Cu at (193.1, 137.6)
- added Q243: 2N3904, Package_TO_SOT_SMD:SOT-23-3, F.Cu at (198.2, 109.9)
- added Q244: 2N3904, Package_TO_SOT_SMD:SOT-23-3, F.Cu at (198.2, 114.5)
- added Q245: 2N3904, Package_TO_SOT_SMD:SOT-23-3, F.Cu at (198.2, 119.1)
- added Q246: 2N3904, Package_TO_SOT_SMD:SOT-23-3, F.Cu at (198.2, 123.8)
- added Q247: 2N3904, Package_TO_SOT_SMD:SOT-23-3, F.Cu at (198.2, 128.4)
- added Q248: 2N3904, Package_TO_SOT_SMD:SOT-23-3, F.Cu at (198.2, 133.0)
- added Q249: 2N3904, Package_TO_SOT_SMD:SOT-23-3, F.Cu at (198.2, 137.6)
- added Q250: 2N3904, Package_TO_SOT_SMD:SOT-23-3, F.Cu at (203.4, 109.9)
- added Q251: 2N3904, Package_TO_SOT_SMD:SOT-23-3, F.Cu at (203.4, 114.5)
- added Q252: 2N3904, Package_TO_SOT_SMD:SOT-23-3, F.Cu at (203.4, 119.1)
- added Q253: 2N3906, Package_TO_SOT_SMD:SOT-23-3, F.Cu at (203.4, 123.8)
- added Q254: 2N3906, Package_TO_SOT_SMD:SOT-23-3, F.Cu at (203.4, 128.4)
- added Q255: 2N3906, Package_TO_SOT_SMD:SOT-23-3, F.Cu at (203.4, 133.0)
- added Q256: 2N3906, Package_TO_SOT_SMD:SOT-23-3, F.Cu at (203.4, 137.6)
- added Q257: 2N3904, Package_TO_SOT_SMD:SOT-23-3, F.Cu at (198.2, -64.8)
- added Q258: 2N3904, Package_TO_SOT_SMD:SOT-23-3, F.Cu at (198.2, -60.2)
- added Q259: 2N3904, Package_TO_SOT_SMD:SOT-23-3, F.Cu at (198.2, -55.6)
- added Q260: 2N3904, Package_TO_SOT_SMD:SOT-23-3, F.Cu at (198.2, -51.0)
- added Q261: 2N3904, Package_TO_SOT_SMD:SOT-23-3, F.Cu at (198.2, -46.3)
- added Q262: 2N3904, Package_TO_SOT_SMD:SOT-23-3, F.Cu at (198.2, -41.7)
- added Q263: 2N3904, Package_TO_SOT_SMD:SOT-23-3, F.Cu at (198.2, -37.1)
- added Q264: 2N3904, Package_TO_SOT_SMD:SOT-23-3, F.Cu at (198.2, -32.5)
- added Q265: 2N3906, Package_TO_SOT_SMD:SOT-23-3, F.Cu at (198.2, -27.8)
- added Q266: 2N3906, Package_TO_SOT_SMD:SOT-23-3, F.Cu at (203.4, -64.8)
- added Q267: 2N3906, Package_TO_SOT_SMD:SOT-23-3, F.Cu at (203.4, -60.2)
- added Q268: 2N3906, Package_TO_SOT_SMD:SOT-23-3, F.Cu at (203.4, -55.6)
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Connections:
- D10 pad 1: /OUT_C1 -> Net-(D10-A)
- D11 pad 3: /OUT_S0 -> Net-(D11-K)
- D3 pad 3: /A0 -> Net-(D3-K)
- D4 pad 3: /B0 -> Net-(D4-K)
- D5 pad 1: Net-(D5-A) -> /alu_5/C1
- D6 pad 1: /~{OUT_G0} -> /alu_5/C2
- D7 pad 1: Net-(D7-A) -> /alu_5/C3
- D7 pad 3: /OUT_P0 -> Net-(D7-K)
- D8 pad 1: Net-(D8-A) -> /C8
- Q1 pad 1: VCC -> 0
- Q1 pad 2: /IN_A0 -> /alu_5/OUT_P0
- Q10 pad 1: 0 -> VCC
- Q10 pad 2: /IN_INV_B -> Net-(Q10-B)
- Q12 pad 2: Net-(Q10-E) -> Net-(Q12-B)
- Q13 pad 2: Net-(D1-K) -> /alu_5/OUT_G0
- Q13 pad 3: Net-(Q11-E) -> Net-(Q13-E)
- Q14 pad 2: Net-(D2-K) -> /alu_5/OUT_G1
- Q14 pad 3: Net-(Q12-E) -> Net-(Q10-E)
- Q15 pad 1: /A0 -> VCC
- Q15 pad 2: Net-(D3-A) -> /alu_5/OUT_G2
- Q15 pad 3: 0 -> Net-(Q11-E)
- Q16 pad 1: /B0 -> VCC
- Q16 pad 2: Net-(D4-A) -> /alu_5/OUT_G3
- Q16 pad 3: 0 -> Net-(Q12-E)
- Q17 pad 2: AND_EN -> /IN_C_IS_1
- Q17 pad 3: Net-(Q17-E) -> Net-(Q13-E)
- Q18 pad 1: 0 -> VCC
- Q18 pad 2: ~{IN_C_IS_0} -> /IN_C_IS_1
- Q18 pad 3: Net-(Q18-E) -> Net-(Q10-E)
- Q19 pad 2: /A0 -> /IN_C_IS_1
- Q19 pad 3: Net-(Q17-E) -> Net-(Q11-E)
- Q2 pad 1: VCC -> 0
- Q2 pad 2: /IN_B0 -> /alu_5/OUT_P1
- Q2 pad 3: Net-(Q2-E) -> Net-(Q10-B)
- Q20 pad 1: 0 -> VCC
- Q20 pad 2: /A0 -> /IN_C_IS_1
- Q20 pad 3: Net-(Q18-E) -> Net-(Q12-E)
- Q21 pad 1: VCC -> Net-(D1-K)
- Q21 pad 2: /B0 -> Net-(D1-A)
- Q21 pad 3: Net-(Q17-E) -> 0
- Q22 pad 1: 0 -> Net-(D2-K)
- Q22 pad 2: /B0 -> Net-(D2-A)
- Q22 pad 3: Net-(Q18-E) -> 0
- Q23 pad 1: Net-(D5-K) -> Net-(D3-K)
- Q23 pad 2: Net-(D5-A) -> Net-(D3-A)
- Q24 pad 1: /~{OUT_G0} -> Net-(D4-K)
- Q24 pad 2: Net-(D6-K) -> Net-(D4-A)
- Q24 pad 3: VCC -> 0
- Q25 pad 1: 0 -> /alu_5/C1
- Q25 pad 2: /A0 -> Net-(D5-K)
- Q25 pad 3: Net-(Q25-E) -> VCC
- Q26 pad 1: 0 -> /alu_5/C2
- Q26 pad 2: /B0 -> Net-(D6-K)
- Q26 pad 3: Net-(Q25-E) -> VCC
- Q27 pad 1: 0 -> /alu_5/C3
- Q27 pad 2: ~{OR_EN} -> Net-(D7-K)
- Q27 pad 3: Net-(Q25-E) -> VCC
- Q28 pad 1: VCC -> /C8
- Q28 pad 2: Net-(Q25-E) -> Net-(D8-K)
- Q28 pad 3: Net-(Q28-E) -> VCC
- Q29 pad 2: Net-(D5-K) -> /A7
- Q29 pad 3: Net-(Q28-E) -> Net-(Q29-E)
- Q3 pad 1: VCC -> 0
- Q3 pad 2: /IN_INV_A -> /alu_5/OUT_P2
- Q3 pad 3: Net-(Q1-E) -> Net-(Q11-B)
- Q30 pad 1: /OUT_P0 -> VCC
- Q30 pad 2: Net-(D7-A) -> /B7
- Q30 pad 3: 0 -> Net-(Q30-E)
- Q31 pad 1: 0 -> VCC
- Q31 pad 2: /IN_C0 -> /IN_INV_A
- Q31 pad 3: Net-(Q31-E) -> Net-(Q29-E)
- Q32 pad 1: 0 -> VCC
- Q32 pad 2: /OUT_P0 -> /IN_INV_B
- Q32 pad 3: Net-(Q31-E) -> Net-(Q30-E)
- Q33 pad 1: VCC -> Net-(D9-K)
- Q33 pad 2: /IN_C0 -> Net-(D9-A)
- Q33 pad 3: Net-(Q33-E) -> 0
- Q34 pad 1: VCC -> Net-(D10-K)
- Q34 pad 2: /OUT_P0 -> Net-(D10-A)
- Q34 pad 3: Net-(Q33-E) -> 0
- Q35 pad 1: Net-(D8-A) -> VCC
- Q35 pad 2: Net-(D8-K) -> /alu_5/C3
- Q35 pad 3: VCC -> Net-(Q35-E)
- Q36 pad 1: Net-(D9-K) -> VCC
- Q36 pad 2: Net-(D9-A) -> /alu_5/OUT_P3
- Q36 pad 3: 0 -> Net-(Q35-E)
- Q37 pad 2: ~{IN_C_IS_1} -> /A7
- Q38 pad 2: /~{OUT_G0} -> /B7
- Q38 pad 3: Net-(Q37-E) -> Net-(Q38-E)
- Q39 pad 2: /IN_C0 -> /IN_INV_A
- Q39 pad 3: Net-(Q39-E) -> Net-(Q37-E)
- Q4 pad 1: VCC -> 0
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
